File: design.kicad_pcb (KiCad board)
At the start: 2 copper layers, 25.8 x 20.2 mm, 0 parts

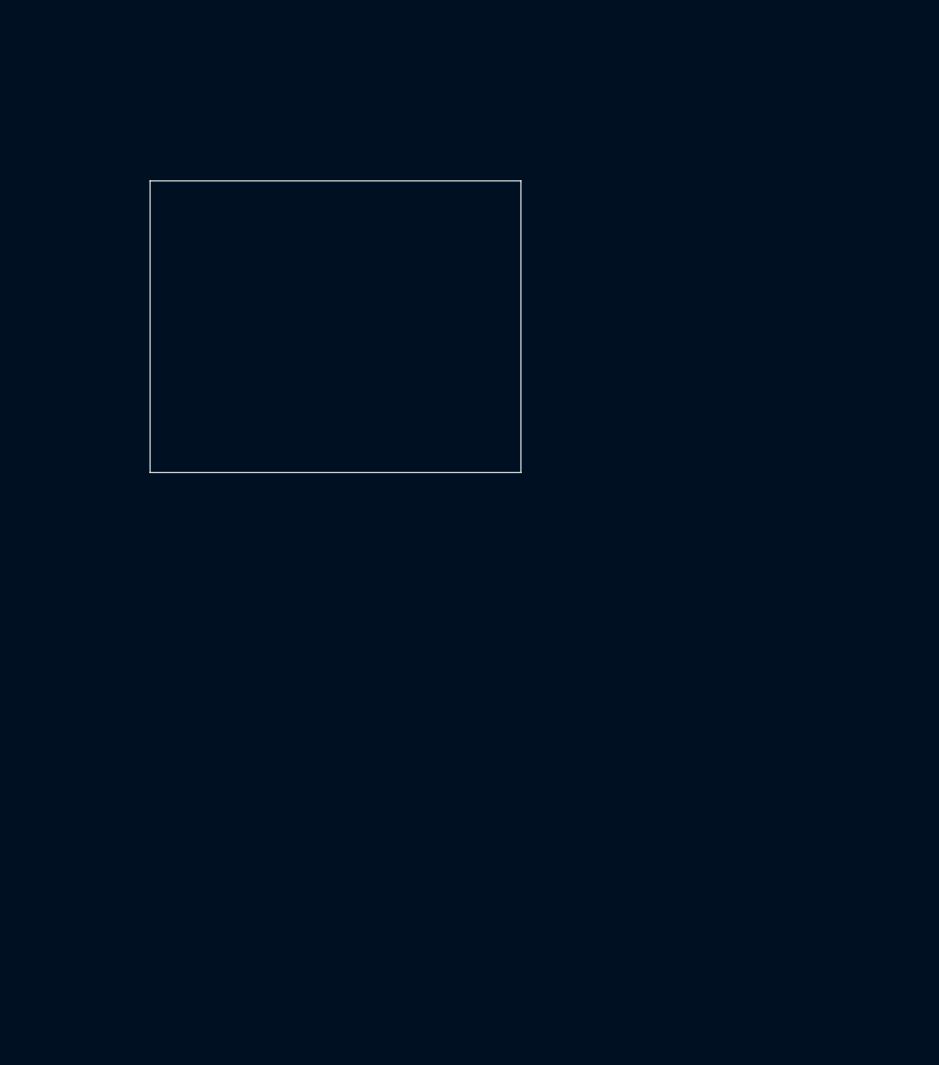
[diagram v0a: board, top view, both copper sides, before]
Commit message: first commit
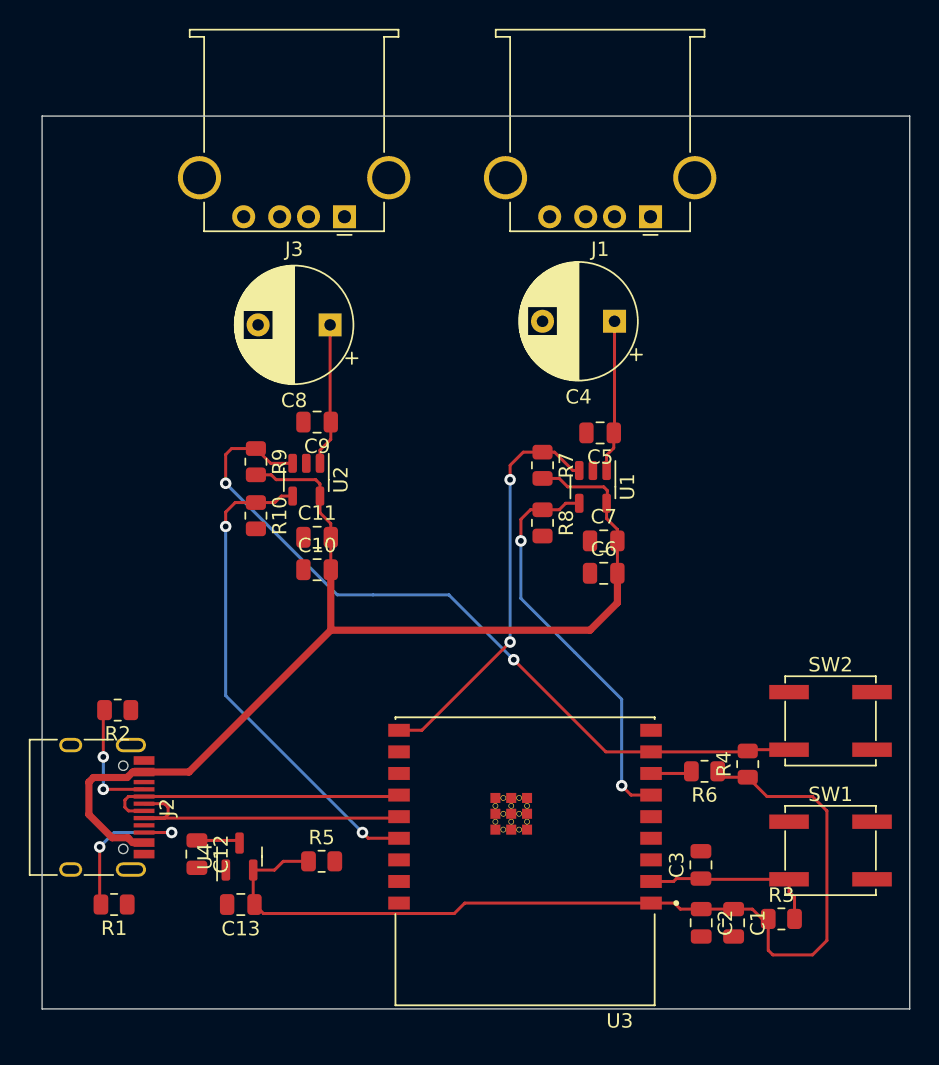
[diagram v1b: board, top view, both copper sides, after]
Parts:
- added C1: 10uF, Capacitor_SMD:C_0805_2012Metric, F.Cu at (172.3, 139.5)
- added C10: 10uF, Capacitor_SMD:C_0805_2012Metric, F.Cu at (143.3, 115.0)
- added C11: 1uF, Capacitor_SMD:C_0805_2012Metric, F.Cu at (143.3, 112.8)
- added C12: 1uF, Capacitor_SMD:C_0805_2012Metric, F.Cu at (135.0, 134.8)
- added C13: 1uF, Capacitor_SMD:C_0805_2012Metric, F.Cu at (138.1, 138.2)
- added C2: 0.1uF, Capacitor_SMD:C_0805_2012Metric, F.Cu at (170.0, 139.5)
- added C3: 1uF, Capacitor_SMD:C_0805_2012Metric, F.Cu at (170.0, 135.5)
- added C4: 120uF, Capacitor_THT:CP_Radial_D8.0mm_P5.00mm, F.Cu at (164.0, 97.8)
- added C5: 0.1uF, Capacitor_SMD:C_0805_2012Metric, F.Cu at (163.0, 105.5)
- added C6: 10uF, Capacitor_SMD:C_0805_2012Metric, F.Cu at (163.2, 115.2)
- added C7: 1uF, Capacitor_SMD:C_0805_2012Metric, F.Cu at (163.2, 113.0)
- added C8: 120uF, Capacitor_THT:CP_Radial_D8.0mm_P5.00mm, F.Cu at (144.2, 98.0)
- added C9: 0.1uF, Capacitor_SMD:C_0805_2012Metric, F.Cu at (143.3, 104.8)
- added J1: USB_A, Connector_USB:USB_A_Stewart_SS-52100-001_Horizontal, F.Cu at (166.5, 90.5)
- added J2: HRO_TYPE-C-31-M-12, Connector_USB:USB_C_Receptacle_HRO_TYPE-C-31-M-12, F.Cu at (127.3, 131.5)
- added J3: USB_A, Connector_USB:USB_A_Stewart_SS-52100-001_Horizontal, F.Cu at (145.2, 90.5)
- added R1: 5.1k, Resistor_SMD:R_0805_2012Metric, F.Cu at (129.2, 138.2)
- added R10: 10k, Resistor_SMD:R_0805_2012Metric, F.Cu at (139.1, 111.2)
- added R2: 5.1k, Resistor_SMD:R_0805_2012Metric, F.Cu at (129.5, 124.8)
- added R3: 10K, Resistor_SMD:R_0805_2012Metric, F.Cu at (175.6, 139.2)
- added R4: 10K, Resistor_SMD:R_0805_2012Metric, F.Cu at (173.2, 128.5)
- added R5: 10K, Resistor_SMD:R_0805_2012Metric, F.Cu at (143.7, 135.2)
- added R6: 10K, Resistor_SMD:R_0805_2012Metric, F.Cu at (170.2, 129.0)
- added R7: 10k, Resistor_SMD:R_0805_2012Metric, F.Cu at (159.0, 107.8)
- added R8: 10k, Resistor_SMD:R_0805_2012Metric, F.Cu at (159.0, 111.8)
- added R9: 10k, Resistor_SMD:R_0805_2012Metric, F.Cu at (139.1, 107.5)
- added SW1: EN, Button_Switch_SMD:SW_SPST_EVPBF, F.Cu at (179.0, 134.5)
- added SW2: IO9, Button_Switch_SMD:SW_SPST_EVPBF, F.Cu at (179.0, 125.5)
- added U1: AP22804AW5, Package_TO_SOT_SMD:SOT-23-5, F.Cu at (162.5, 109.2)
- added U2: AP22804AW5, Package_TO_SOT_SMD:SOT-23-5, F.Cu at (142.6, 108.8)
- added U3: ESP32-C3-WROOM-02-N4, MCU_Espressif_custom:MODULE_ESP32-C3-WROOM-02-H4, F.Cu at (157.8, 135.2)
- added U4: MCP1700T-3302E, Package_TO_SOT_SMD:SOT-23, F.Cu at (138.0, 134.9)
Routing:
- net VCC: track 0.00 -> 80.2 mm
- net +3.3V: track 0.00 -> 67.7 mm
- net IO9: track 0.00 -> 54.1 mm, vias 0 -> 2
- net IO3: track 0.00 -> 34.0 mm, vias 0 -> 2
- net I010: track 0.00 -> 28.2 mm, vias 0 -> 2
- net IO7: track 0.00 -> 28.2 mm, vias 0 -> 2
- net D+: track 0.00 -> 21.8 mm
- net D-: track 0.00 -> 21.1 mm
- net /EN: track 0.00 -> 12.6 mm
- net /CC2: track 0.00 -> 11.4 mm, vias 0 -> 2
- net USB1_VCC: track 0.00 -> 10.6 mm
- net USB2_VCC: track 0.00 -> 9.94 mm
- net /CC1: track 0.00 -> 8.37 mm, vias 0 -> 2
- net IO8: track 0.00 -> 2.86 mm
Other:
- board size 25.8 x 20.2 mm -> 60.2 x 62 mm
